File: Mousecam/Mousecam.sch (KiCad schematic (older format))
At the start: 0 parts

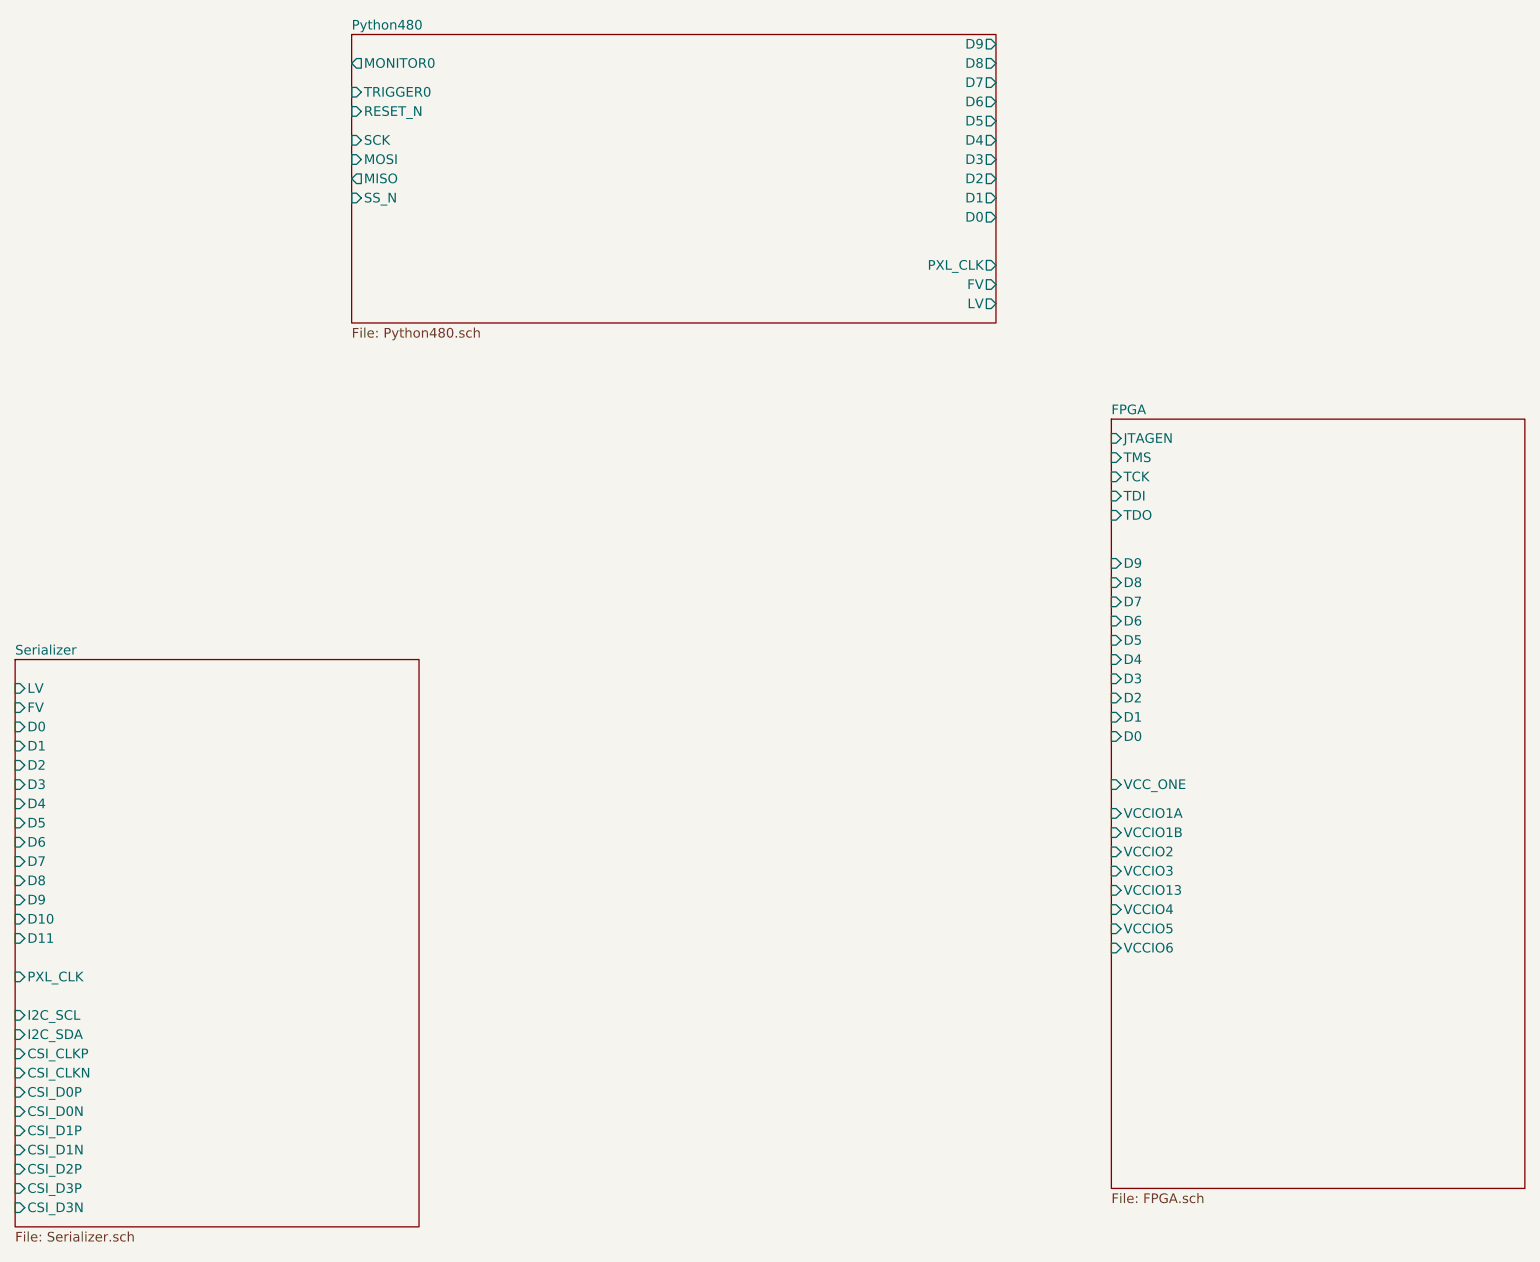
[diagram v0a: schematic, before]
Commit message: sync
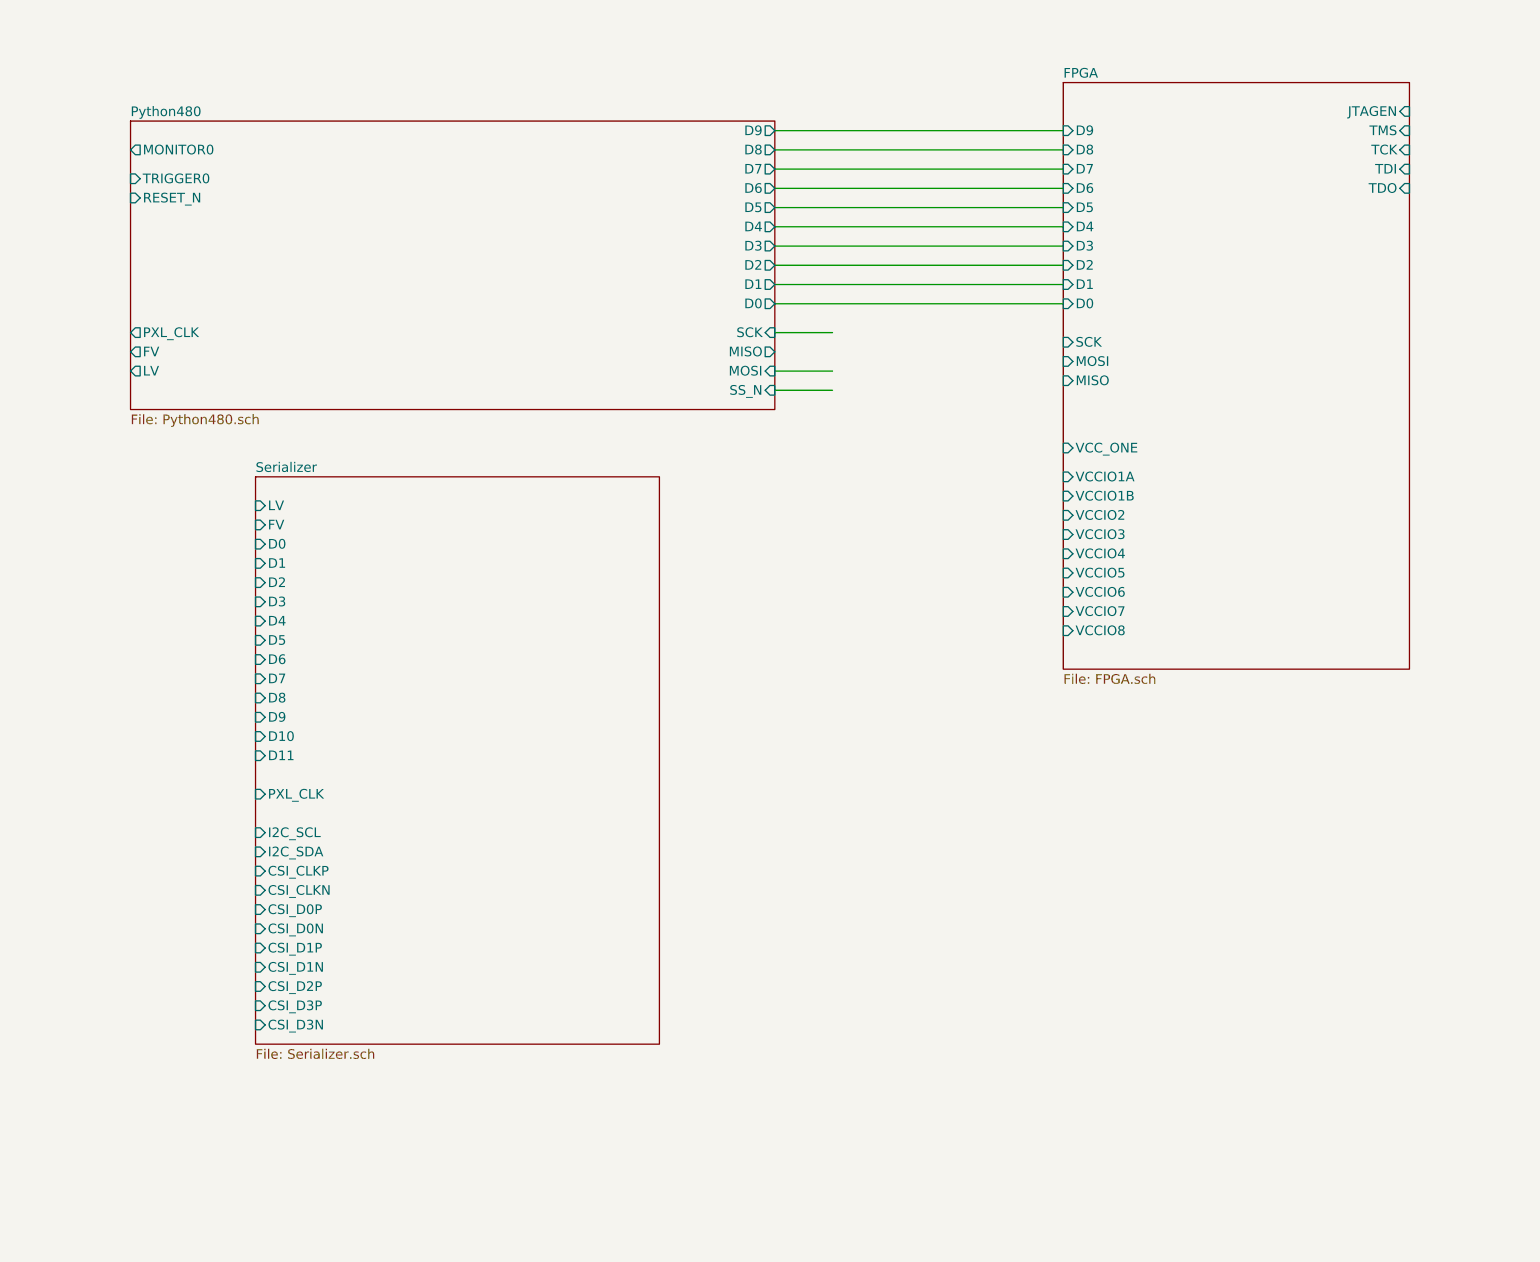
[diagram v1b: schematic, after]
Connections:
- wire segments 0 -> 13
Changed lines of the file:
@@
 $EndDescr
 $Sheet
-S 2950 900  3350 1500
+S 1800 1350 3350 1500
 U 607CBC7A
 F0 "Python480" 50
 F1 "Python480.sch" 50
-F2 "MONITOR0" O L 2950 1050 50
-F3 "TRIGGER0" I L 2950 1200 50
-F4 "RESET_N" I L 2950 1300 50
-F5 "SCK" I L 2950 1450 50
-F6 "MOSI" I L 2950 1550 50
-F7 "MISO" O L 2950 1650 50
-F8 "SS_N" I L 2950 1750 50
-F9 "D9" O R 6300 950 50
-F10 "D8" O R 6300 1050 50
-F11 "D7" O R 6300 1150 50
-F12 "D6" O R 6300 1250 50
-F13 "D5" O R 6300 1350 50
-F14 "D4" O R 6300 1450 50
-F15 "LV" O R 6300 2300 50
-F16 "FV" O R 6300 2200 50
-F17 "PXL_CLK" O R 6300 2100 50
-F18 "D3" O R 6300 1550 50
-F19 "D2" O R 6300 1650 50
-F20 "D1" O R 6300 1750 50
-F21 "D0" O R 6300 1850 50
+F2 "MONITOR0" O L 1800 1500 50
+F3 "TRIGGER0" I L 1800 1650 50
+F4 "RESET_N" I L 1800 1750 50
+F5 "SCK" I R 5150 2450 50
+F6 "MOSI" I R 5150 2650 50
+F7 "MISO" O R 5150 2550 50
+F8 "SS_N" I R 5150 2750 50
+F9 "D9" O R 5150 1400 50
+F10 "D8" O R 5150 1500 50
+F11 "D7" O R 5150 1600 50
+F12 "D6" O R 5150 1700 50
+F13 "D5" O R 5150 1800 50
+F14 "D4" O R 5150 1900 50
+F15 "LV" O L 1800 2650 50
+F16 "FV" O L 1800 2550 50
+F17 "PXL_CLK" O L 1800 2450 50
+F18 "D3" O R 5150 2000 50
+F19 "D2" O R 5150 2100 50
+F20 "D1" O R 5150 2200 50
+F21 "D0" O R 5150 2300 50
 $EndSheet
 $Sheet
-S 1200 4150 2100 2950
+S 2450 3200 2100 2950
 U 607CBDDC
 F0 "Serializer" 50
 F1 "Serializer.sch" 50
-F2 "LV" I L 1200 4300 50
-F3 "FV" I L 1200 4400 50
-F4 "D0" I L 1200 4500 50
-F5 "D1" I L 1200 4600 50
-F6 "D2" I L 1200 4700 50
-F7 "D3" I L 1200 4800 50
-F8 "D4" I L 1200 4900 50
-F9 "D5" I L 1200 5000 50
-F10 "D6" I L 1200 5100 50
-F11 "D7" I L 1200 5200 50
-F12 "D8" I L 1200 5300 50
-F13 "D9" I L 1200 5400 50
-F14 "I2C_SCL" I L 1200 6000 50
-F15 "D10" I L 1200 5500 50
-F16 "D11" I L 1200 5600 50
-F17 "PXL_CLK" I L 1200 5800 50
-F18 "I2C_SDA" I L 1200 6100 50
-F19 "CSI_CLKP" I L 1200 6200 50
-F20 "CSI_CLKN" I L 1200 6300 50
-F21 "CSI_D0P" I L 1200 6400 50
-F22 "CSI_D0N" I L 1200 6500 50
-F23 "CSI_D1P" I L 1200 6600 50
-F24 "CSI_D1N" I L 1200 6700 50
-F25 "CSI_D2P" I L 1200 6800 50
-F26 "CSI_D3P" I L 1200 6900 50
-F27 "CSI_D3N" I L 1200 7000 50
+F2 "LV" I L 2450 3350 50
+F3 "FV" I L 2450 3450 50
+F4 "D0" I L 2450 3550 50
+F5 "D1" I L 2450 3650 50
+F6 "D2" I L 2450 3750 50
+F7 "D3" I L 2450 3850 50
+F8 "D4" I L 2450 3950 50
+F9 "D5" I L 2450 4050 50
+F10 "D6" I L 2450 4150 50
+F11 "D7" I L 2450 4250 50
+F12 "D8" I L 2450 4350 50
+F13 "D9" I L 2450 4450 50
+F14 "I2C_SCL" I L 2450 5050 50
+F15 "D10" I L 2450 4550 50
+F16 "D11" I L 2450 4650 50
+F17 "PXL_CLK" I L 2450 4850 50
+F18 "I2C_SDA" I L 2450 5150 50
+F19 "CSI_CLKP" I L 2450 5250 50
+F20 "CSI_CLKN" I L 2450 5350 50
+F21 "CSI_D0P" I L 2450 5450 50
+F22 "CSI_D0N" I L 2450 5550 50
+F23 "CSI_D1P" I L 2450 5650 50
+F24 "CSI_D1N" I L 2450 5750 50
+F25 "CSI_D2P" I L 2450 5850 50
+F26 "CSI_D3P" I L 2450 5950 50
+F27 "CSI_D3N" I L 2450 6050 50
 $EndSheet
 $Sheet
-S 6900 2900 2150 4000
+S 6650 1150 1800 3050
 U 607CBD48
 F0 "FPGA" 50
 F1 "FPGA.sch" 50
-F2 "JTAGEN" I L 6900 3000 50
-F3 "TMS" I L 6900 3100 50
-F4 "TCK" I L 6900 3200 50
-F5 "TDI" I L 6900 3300 50
-F6 "TDO" I L 6900 3400 50
-F7 "D9" I L 6900 3650 50
-F8 "D8" I L 6900 3750 50
-F9 "D7" I L 6900 3850 50
-F10 "D6" I L 6900 3950 50
-F11 "D5" I L 6900 4050 50
-F12 "D4" I L 6900 4150 50
-F13 "D3" I L 6900 4250 50
-F14 "D2" I L 6900 4350 50
-F15 "D1" I L 6900 4450 50
-F16 "D0" I L 6900 4550 50
-F17 "VCC_ONE" I L 6900 4800 50
-F18 "VCCIO1A" I L 6900 4950 50
-F19 "VCCIO1B" I L 6900 5050 50
-F20 "VCCIO2" I L 6900 5150 50
-F21 "VCCIO3" I L 6900 5250 50
-F22 "VCCIO13" I L 6900 5350 50
-F23 "VCCIO4" I L 6900 5450 50
-F24 "VCCIO5" I L 6900 5550 50
-F25 "VCCIO6" I L 6900 5650 50
+F2 "D9" I L 6650 1400 50
+F3 "D8" I L 6650 1500 50
+F4 "D7" I L 6650 1600 50
+F5 "D6" I L 6650 1700 50
+F6 "D5" I L 6650 1800 50
+F7 "D4" I L 6650 1900 50
+F8 "D3" I L 6650 2000 50
+F9 "D2" I L 6650 2100 50
+F10 "D1" I L 6650 2200 50
+F11 "D0" I L 6650 2300 50
+F12 "VCC_ONE" I L 6650 3050 50
+F13 "VCCIO1A" I L 6650 3200 50
+F14 "VCCIO1B" I L 6650 3300 50
+F15 "VCCIO2" I L 6650 3400 50
+F16 "VCCIO4" I L 6650 3600 50
+F17 "VCCIO5" I L 6650 3700 50
+F18 "VCCIO6" I L 6650 3800 50
+F19 "VCCIO7" I L 6650 3900 50
+F20 "VCCIO8" I L 6650 4000 50
+F21 "VCCIO3" I L 6650 3500 50
+F22 "JTAGEN" I R 8450 1300 50
+F23 "TMS" I R 8450 1400 50
+F24 "TCK" I R 8450 1500 50
+F25 "TDI" I R 8450 1600 50
+F26 "TDO" I R 8450 1700 50
+F27 "SCK" I L 6650 2500 50
+F28 "MOSI" I L 6650 2600 50
+F29 "MISO" I L 6650 2700 50
 $EndSheet
+Wire Wire Line
+	5150 2450 5450 2450
+Wire Wire Line
+	5150 2650 5450 2650
+Wire Wire Line
+	5150 2750 5450 2750
+Wire Wire Line
+	5150 1400 6650 1400
+Wire Wire Line
+	5150 1500 6650 1500
+Wire Wire Line
+	5150 1600 6650 1600
+Wire Wire Line
+	5150 1700 6650 1700
+Wire Wire Line
+	5150 1800 6650 1800
+Wire Wire Line
+	5150 1900 6650 1900
+Wire Wire Line
+	5150 2000 6650 2000
+Wire Wire Line
+	5150 2100 6650 2100
+Wire Wire Line
+	5150 2200 6650 2200
+Wire Wire Line
+	5150 2300 6650 2300
 $EndSCHEMATC
